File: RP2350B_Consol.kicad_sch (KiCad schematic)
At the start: 50 parts, among them J1 Conn_01x15_Socket, J10 VGA, J11 NES_Joystick1, J12 NES_Joystick2, J2 Conn_01x15_Socket, J3 Conn_01x15_Socket, J4 Conn_01x15_Socket, J5 Conn_02x06_Odd_Even, J6 Conn_02x20_Odd_Even, J7 Conn_02x06_Odd_Even, J8 Conn_02x20_Odd_Even, J9 PJ320D, SW1 "RESET", U3 SN76489AN

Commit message: Update RP2350B_Consol.kicad_sch
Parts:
- removed C1: 0.1uF, Capacitor_SMD:C_0805_2012Metric_Pad1.18x1.45mm_HandSolder, symbol Device:C_Small
- removed C4: 0.1µF, Capacitor_SMD:C_0805_2012Metric_Pad1.18x1.45mm_HandSolder, symbol Device:C
- removed J11: NES_Joystick1, Connector_Dsub:DSUB-9_Male_Vertical_P2.77x2.84mm_MountingHoles, symbol Connector:DE9_Plug_MountingHoles
- removed J12: NES_Joystick2, Connector_Dsub:DSUB-9_Male_Vertical_P2.77x2.84mm_MountingHoles, symbol Connector:DE9_Plug_MountingHoles
- removed J7: Conn_02x06_Odd_Even, UM6502:EDGE_2x12, symbol Connector_Generic:Conn_02x06_Odd_Even
- removed J8: Conn_02x20_Odd_Even, UM6502:EDGE_2x20, symbol Connector_Generic:Conn_02x20_Odd_Even
- removed R1, R2, R3, R4: 1k, symbol Device:R_Small
- removed R10, R11, R12, R5, R6, R7, R8, R9: 33, symbol Device:R_Small
- removed R17, R19: 1k, Resistor_SMD:R_0805_2012Metric_Pad1.20x1.40mm_HandSolder, symbol Device:R
- removed R18: 3.9k, Resistor_SMD:R_0805_2012Metric_Pad1.20x1.40mm_HandSolder, symbol Device:R
- removed R20, R22, R24: 2k, Resistor_SMD:R_0805_2012Metric_Pad1.20x1.40mm_HandSolder, symbol Device:R
- removed R21, R23, R25: 510, Resistor_SMD:R_0805_2012Metric_Pad1.20x1.40mm_HandSolder, symbol Device:R
- removed R26, R27: 100, Resistor_SMD:R_0805_2012Metric_Pad1.20x1.40mm_HandSolder, symbol Device:R
- removed SW1: "RESET", symbol Switch:SW_Push
- removed U1: ~, Package_DIP:DIP-40_W15.24mm_Socket, symbol 6502:UM6502
- removed U3: SN76489AN, Package_DIP:DIP-16_W7.62mm_LongPads, symbol LeakoChips:SN76489AN
- removed u2: ~, RP2350B_WeAct:RP2350B_WeAct, symbol RP2350B:RP2350BSYM
- added C1: 6800, Capacitor_SMD:C_0805_2012Metric_Pad1.18x1.45mm_HandSolder, symbol Device:C
- added J7: NES_Joystick1, Connector_Dsub:DSUB-9_Male_Vertical_P2.77x2.84mm_MountingHoles, symbol Connector:DE9_Plug_MountingHoles
- added J8: NES_Joystick2, Connector_Dsub:DSUB-9_Male_Vertical_P2.77x2.84mm_MountingHoles, symbol Connector:DE9_Plug_MountingHoles
- added R1: 100, Resistor_SMD:R_0805_2012Metric_Pad1.20x1.40mm_HandSolder, symbol Device:R
- added R10, R12: 510, Resistor_SMD:R_0805_2012Metric_Pad1.20x1.40mm_HandSolder, symbol Device:R
- added R11, R9: 2k, Resistor_SMD:R_0805_2012Metric_Pad1.20x1.40mm_HandSolder, symbol Device:R
- added R2, R4, R6, R8: 1k, Resistor_SMD:R_0805_2012Metric_Pad1.20x1.40mm_HandSolder, symbol Device:R
- added R3, R5, R7: 3.9k, Resistor_SMD:R_0805_2012Metric_Pad1.20x1.40mm_HandSolder, symbol Device:R
- added SW1: RotaryEncoder_for_Coleco_20imp, symbol Device:RotaryEncoder
- added U2: SN76489AN, Package_DIP:DIP-16_W7.62mm_LongPads, symbol LeakoChips:SN76489AN
- added u1: ~, RP2350B_WeAct:RP2350B_WeAct, symbol RP2350B:RP2350BSYM
- C2: value 6800 -> 1.0uF
- C3: value 1.0µF -> 0.1uF
- R13: value 1kΩ -> 2k; DigiKey RMCF0805FT1K00CT-ND -> RMCF0805JT100RCT-ND
- R14: value 3.9k -> 510
- R15: value 1k -> 100; DigiKey RMCF0805JT100RCT-ND -> (none)
- R16: value 3.9k -> 100; DigiKey RMCF0805JT100RCT-ND -> (none)
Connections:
- net DA0 is gone; now on net D0: J4.14 (Pin_14), J6.22 (Pin_22)
- net DA1 is gone; now on net D1: J3.15 (Pin_15), J6.21 (Pin_21)
- net DA2 is gone; now on net D2: J4.15 (Pin_15), J6.20 (Pin_20)
- net DA3 is gone; now on net D3: J1.15 (Pin_15), J6.19 (Pin_19)
- net DA4 is gone; now on net D4: J2.15 (Pin_15), J6.18 (Pin_18)
- net DA5 is gone; now on net D5: J1.14 (Pin_14), J6.17 (Pin_17)
- net DA6 is gone; now on net D6: J2.14 (Pin_14), J6.16 (Pin_16)
- net DA7 is gone; now on net D7: J1.13 (Pin_13), J6.15 (Pin_15)
- net +5V: now also C3.2, R1.1, U2.16 (Vcc)
- net 5V: now also J7.6, J8.6
- net Audio_Out: now also R2.1, U2.7 (Audio); no longer R13.1
- net B: now also R13.2, R14.2, R7.2, R8.2
- net CLK_VDP: now also J5.3 (Pin_3)
- net D0: now also U2.10 (D7)
- net D1: now also U2.11 (D6)
- net D2: now also U2.12 (D5)
- net D3: now also U2.13 (D4)
- net D4: now also U2.15 (D3)
- net D5: now also U2.1 (D2)
- net D6: now also U2.2 (D1)
- net D7: now also U2.3 (D0)
- net G: now also R11.2, R12.2, R5.2, R6.2; no longer R16.2
- net GND: now also C3.1, C1.2, J7.0 (PAD), J7.8, J8.0 (PAD), J8.8, U2.8 (GND); no longer C2.2
- net GP35: now also U2.4 (READY), U2.5 (~{WE})
- net GP41: now also U2.6 (~{CE})
- net GP42: now also J7.4, J8.4
- net GP43: now also J7.3, J8.3
- net GP44: now also J7.2
- net GP45: now also J8.2
- net HSYNC: now also R15.2
- net R: now also R10.2, R3.2, R4.2, R9.2; no longer R14.2, R15.2
- net VSYNC: now also R16.2
- net at J10.13: now also R15.1
- net at J10.14: now also R16.1
- net at FB1.1: now also C2.1; no longer C3.1
- net at DD1.8 (GP6): now also R5.1; no longer R16.1
- net at DD1.13 (GP11): now also R13.1
- net CLK_PSG: now reaches J5.4 (Pin_4)
- net CLK_PSG: now also U2.14 (CLK)
- net ~{RESET}: now reaches J6.3 (Pin_3)
- net ~{RESET}: now also DD1.26 (GP23)
- net at DD1.12 (GP10): now also R7.1
- net at DD1.11 (GP9): now also R12.1
- net at DD1.14 (GP12): now also R8.1
- net at DD1.10 (GP8): now also R6.1
- net at DD1.16 (GP13): now also R14.1
- net at DD1.3 (GP2): now also R3.1; no longer R14.1
- net at DD1.4 (GP3): now also R9.1
- net at DD1.5 (GP4): now also R4.1; no longer R15.1
- net at DD1.7 (GP5): now also R10.1
- net at DD1.9 (GP7): now also R11.1
- net A1 renamed GP7
- net A10 renamed GP16
- net A11 renamed GP17
- net A12 renamed GP18
- net A13 renamed GP19
- net A14 renamed GP20
- net A15 renamed GP21
- net A2 renamed GP8
- net A3 renamed GP9
- net A4 renamed GP10
- net A5 renamed GP11
- net A6 renamed GP12
- net A7 renamed GP13
- net A8 renamed GP14
- net A9 renamed GP15
- net CLK renamed GP37
- net CLK_2MHz renamed GP34
- net F1 renamed GP32
- net F2 renamed GP33
- net GP46 renamed Encoder_A
- net Encoder_A: now also SW1.A
- net GP47 renamed Encoder_B
- net Encoder_B: now also SW1.B; no longer DD1.26 (GP23)
- new net: C1.1, C2.2, R2.2
- new net: R1.2, SW1.C
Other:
- added sheet MOC6502 (MOC6502.kicad_sch)
- added sheet Z80 (Z80.kicad_sch)
- note added: "https://github.com/visrealm/pico9918"

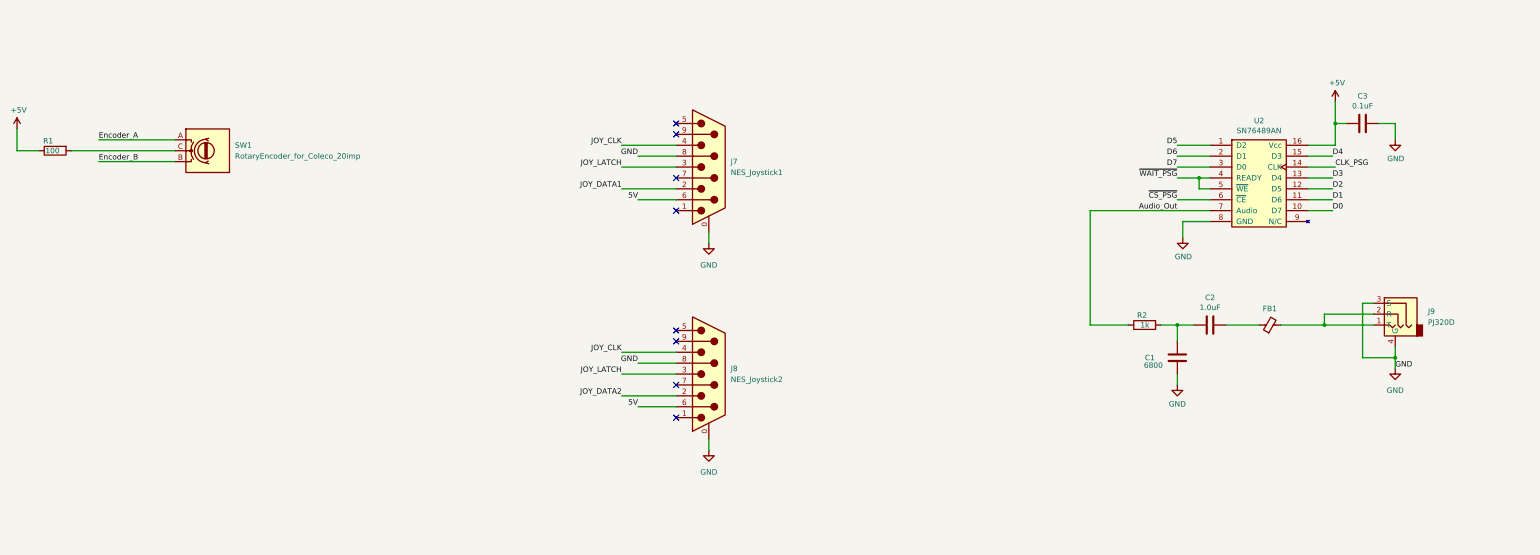
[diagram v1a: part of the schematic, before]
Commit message: Update RP2350B_Consol.kicad_sch
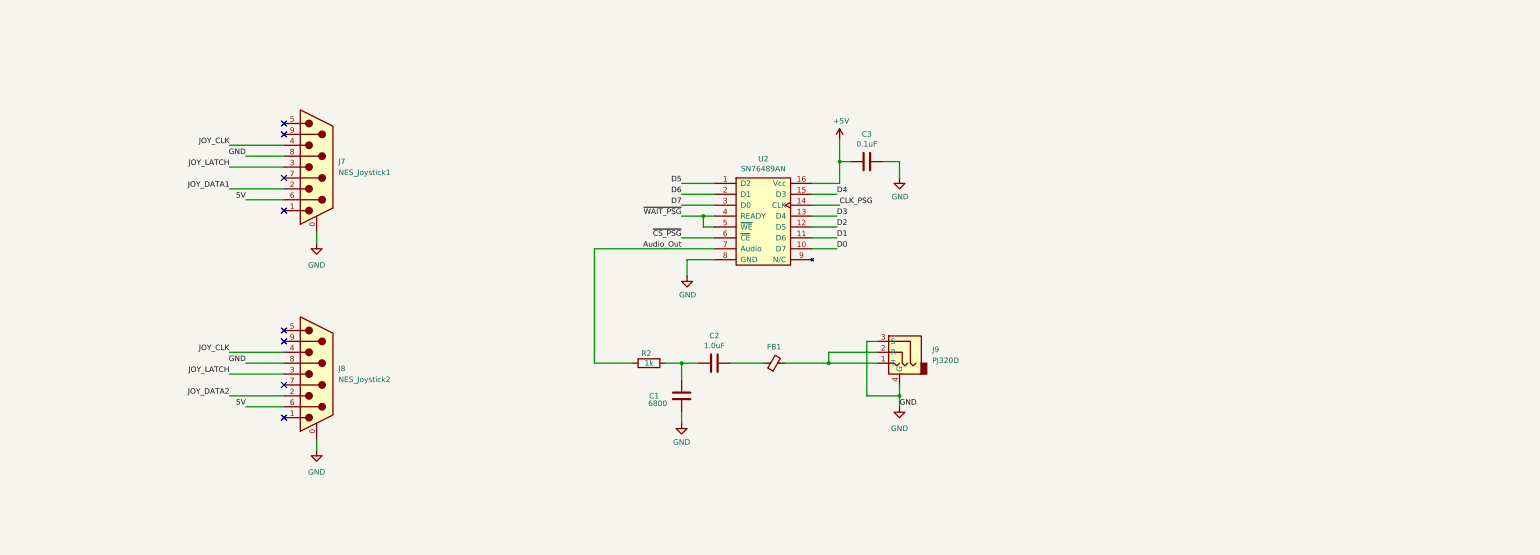
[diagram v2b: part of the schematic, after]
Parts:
- removed R1: 100, Resistor_SMD:R_0805_2012Metric_Pad1.20x1.40mm_HandSolder, symbol Device:R
- removed SW1: RotaryEncoder_for_Coleco_20imp, symbol Device:RotaryEncoder
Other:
- moved on the sheet: C1, C2, C3, FB1, J7, J8, J9, R2, U2
